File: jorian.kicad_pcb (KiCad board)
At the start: 2 copper layers, 98.9 x 100 mm, 90 parts, among them J6 lipo_charger, U3 LP3990-3.3v

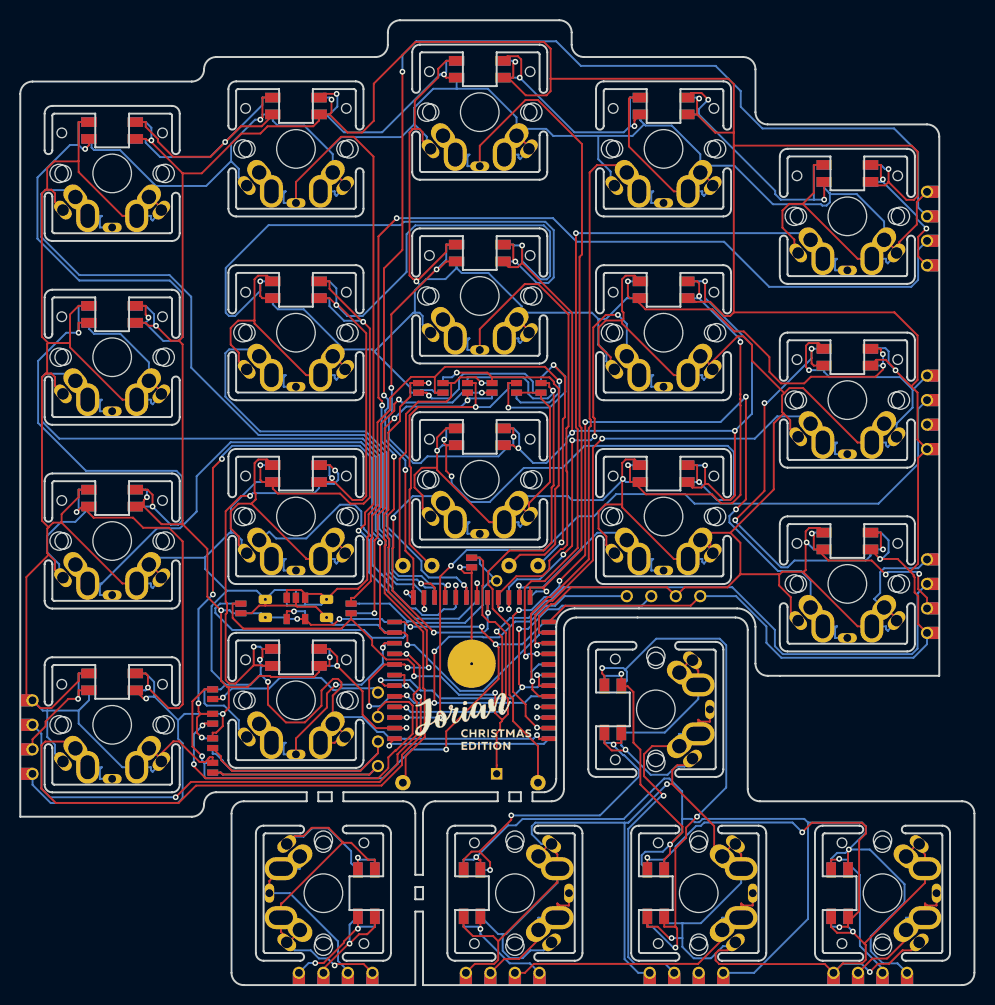
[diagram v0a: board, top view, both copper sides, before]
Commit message: reroute take 3, moved a bit by hand
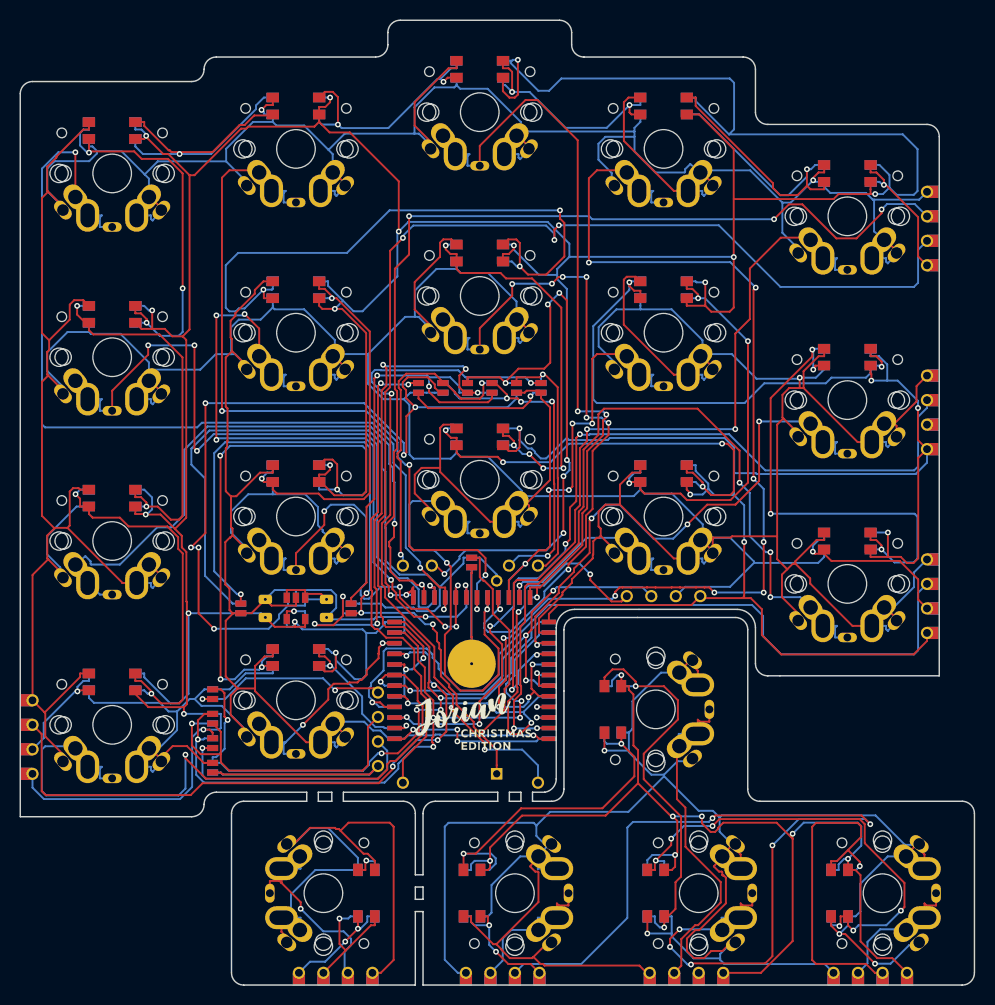
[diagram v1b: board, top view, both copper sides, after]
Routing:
- net /S20_B: track 32.5 -> 99.3 mm, vias 0 -> 6
- net /S4: track 72.6 -> 118.2 mm, vias 1 -> 11
- net BAT-: track 63.8 -> 100.2 mm, vias 2 -> 4
- net BAT+: track 48.5 -> 79.4 mm
- net OUT+: track 65.3 -> 94.9 mm, vias 1 -> 6
- net /GND_B: track 216.0 -> 244.3 mm, vias 5 -> 4
- net Net-(J6-Pad4): track 32.8 -> 60.9 mm, vias 1 -> 7
- net VCC: track 611.7 -> 635.6 mm
- net /S19: track 128.2 -> 105.7 mm, vias 4 -> 5
- net LIPO+: track 35.8 -> 56.7 mm, vias 3 -> 6
- net /DIN21_B: track 18.1 -> 38.1 mm
- net SCL: track 90.9 -> 71.4 mm, vias 6 -> 5
- net Net-(L12-Pad3): track 44.0 -> 62.9 mm, vias 3 -> 4
- net /VCC_B: track 139.9 -> 122.5 mm, vias 4 -> 7
- net /S7: track 55.6 -> 72.8 mm, vias 1 -> 6
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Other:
- outline, holes or cut-outs redrawn
